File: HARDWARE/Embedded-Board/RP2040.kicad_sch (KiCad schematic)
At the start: 25 parts, among them J6 GPIO PINS, SW5 BOOT, U2 W25Q16JVS, U3 RP2040, Y1 12MHz

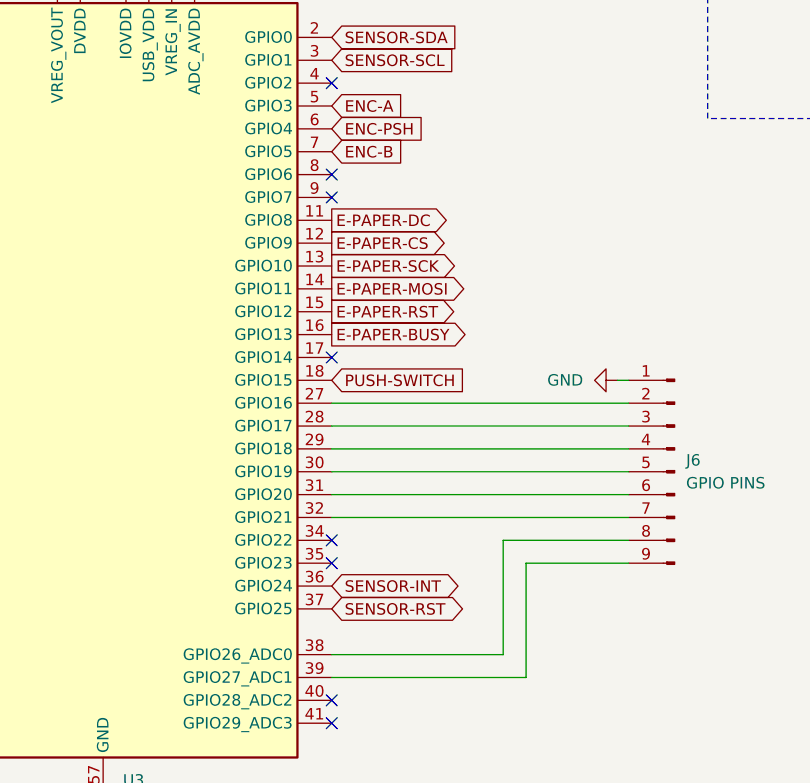
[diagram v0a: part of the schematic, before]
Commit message: Final PCB version
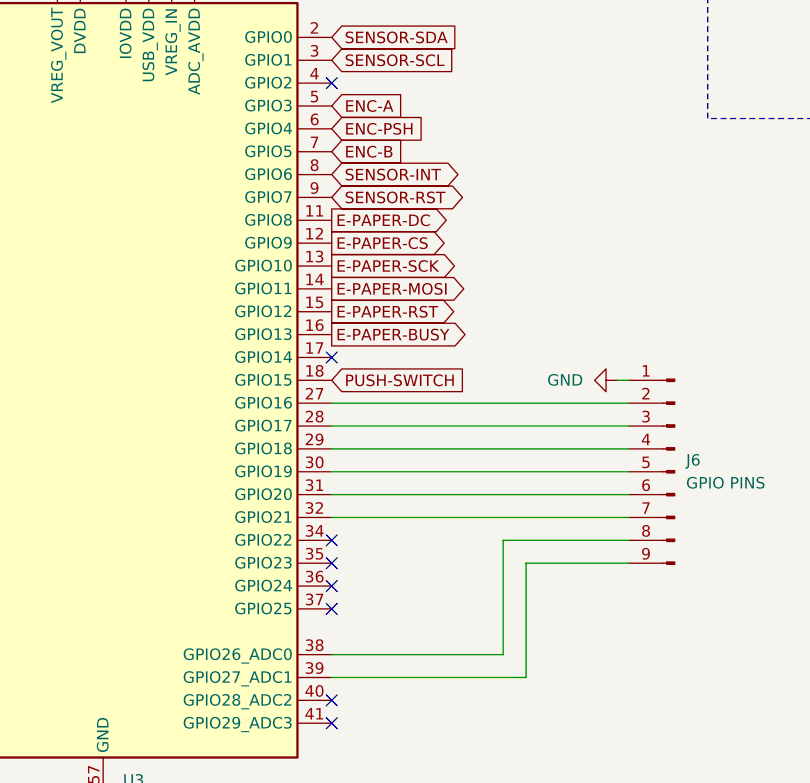
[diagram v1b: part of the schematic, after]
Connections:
- net SENSOR-INT: now also U3.8 (GPIO6); no longer U3.36 (GPIO24)
- net SENSOR-RST: now also U3.9 (GPIO7); no longer U3.37 (GPIO25)
